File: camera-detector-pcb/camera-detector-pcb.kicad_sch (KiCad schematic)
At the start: 29 parts, among them J1 Conn_01x07, J2 Conn_01x07, J3 Conn_01x04, Q1 PN2222A, SW1 SW_Push, SW2 SW_Push, SW3 SW_Wuerth_450301014042, SW4 SW_Push, U1 74AHCT125

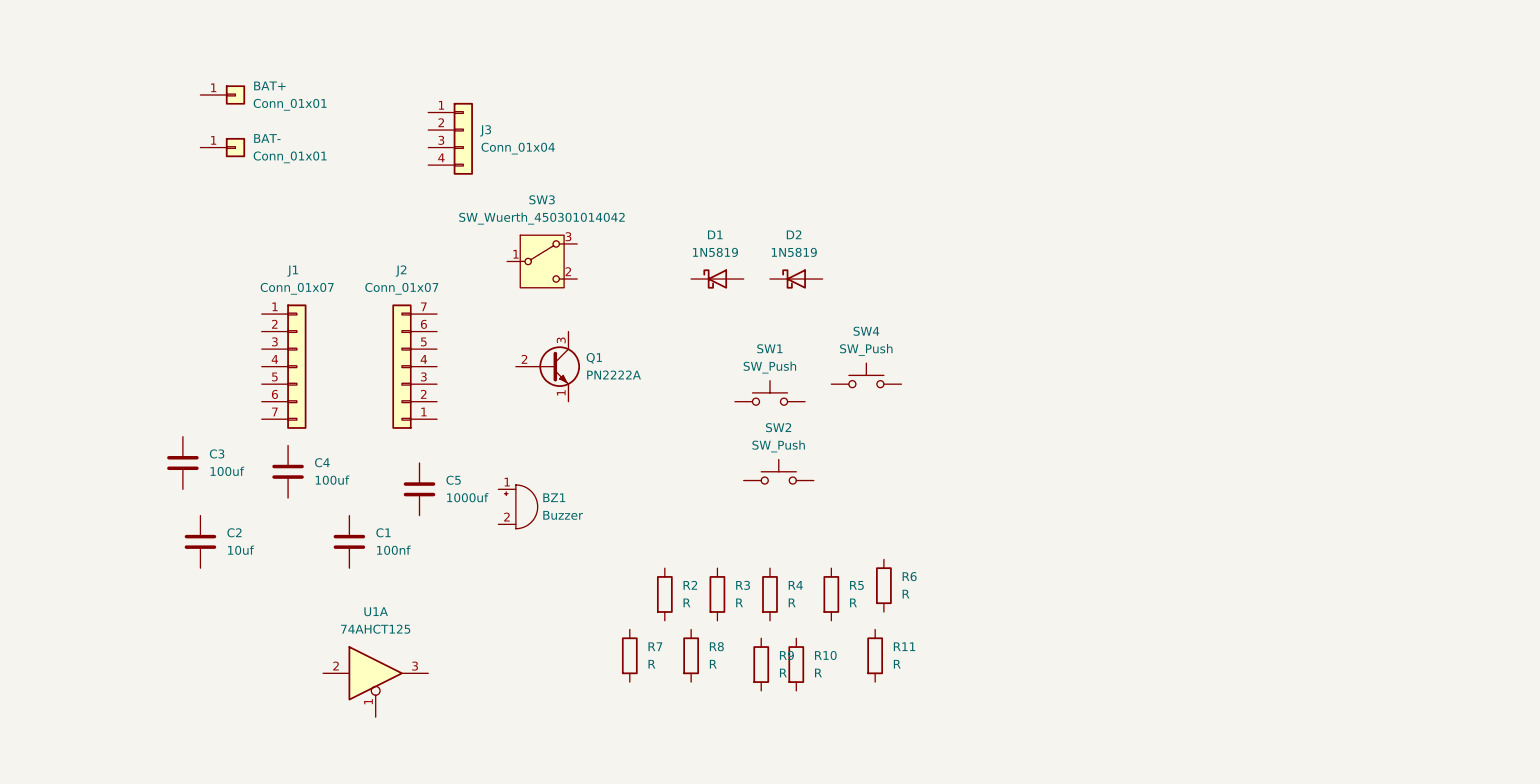
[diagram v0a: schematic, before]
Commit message: completed schematic
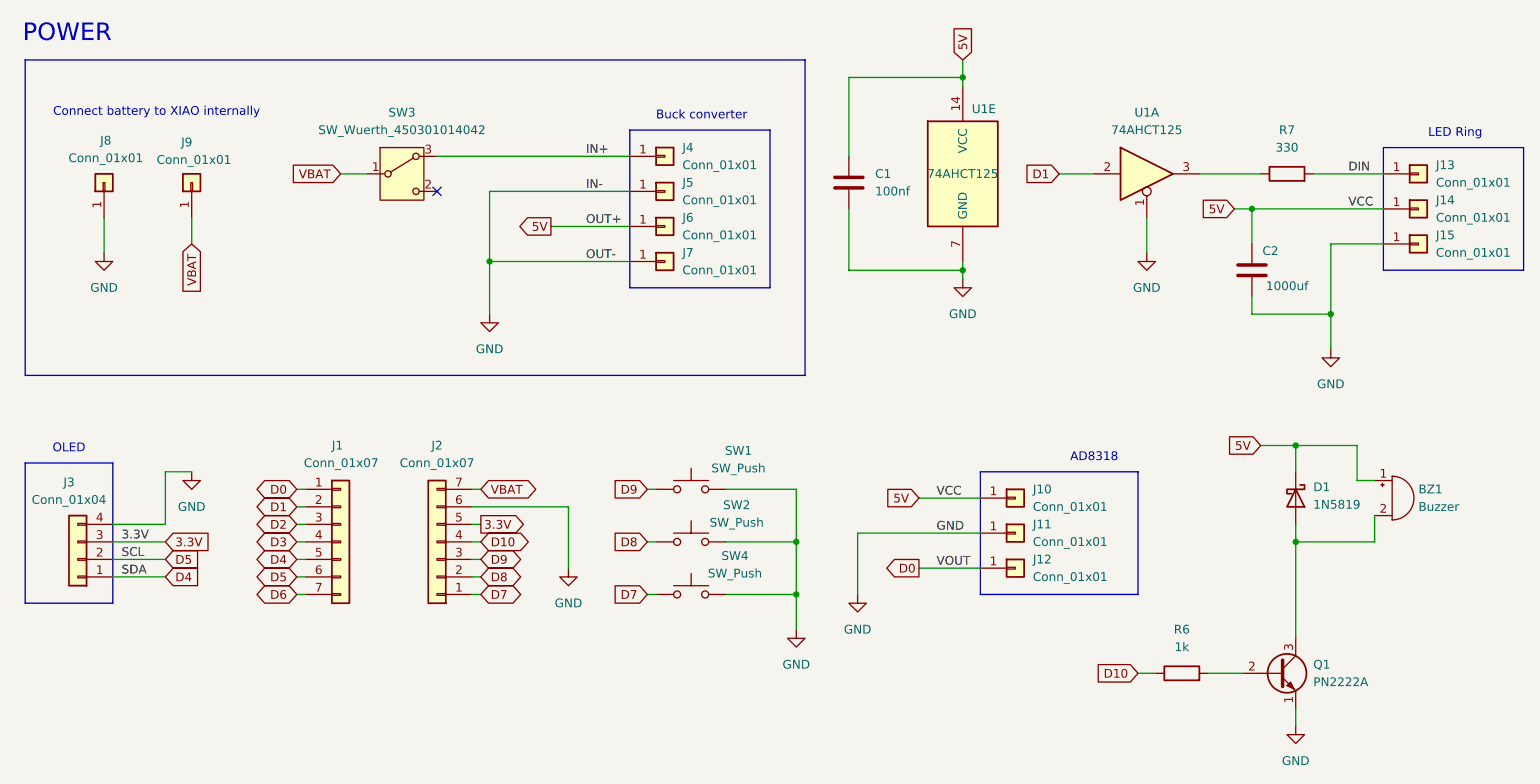
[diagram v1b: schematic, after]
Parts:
- removed C3, C4: 100uf, Capacitor_THT:C_Radial_D5.0mm_H7.0mm_P2.00mm, symbol Device:C
- removed C5: 1000uf, Capacitor_THT:C_Radial_D8.0mm_H11.5mm_P3.50mm, symbol Device:C
- removed D2: 1N5819, Diode_THT:D_DO-41_SOD81_P10.16mm_Horizontal, symbol Diode:1N5819
- removed R10, R11, R2, R3, R4, R5, R8, R9: R, Resistor_THT:R_Axial_DIN0207_L6.3mm_D2.5mm_P15.24mm_Horizontal, symbol Device:R
- added J10, J11, J12, J13, J14, J15, J4, J5, J6, J7: Conn_01x01, symbol Connector_Generic:Conn_01x01
- added unit 5 of U1
- C1: footprint Capacitor_THT:C_Disc_D4.7mm_W2.5mm_P5.00mm -> Capacitor_THT:C_Disc_D3.0mm_W1.6mm_P2.50mm
- C2: value 10uf -> 1000uf; footprint Capacitor_THT:C_Radial_D8.0mm_H7.0mm_P3.50mm -> Capacitor_THT:CP_Radial_D10.0mm_P5.00mm
- R6: value R -> 1k
- R7: value R -> 330
- U1: footprint Package_DIP:DIP-14_W7.62mm -> (none)
- renumbered BAT- to J8, BAT+ to J9
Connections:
- net VBAT: now reaches SW3.1 (B)
- net VBAT: now also J2.7 (Pin_7), J9.1 (Pin_1)
- net IN+: now reaches SW3.3 (A)
- net IN+: now also J4.1 (Pin_1)
- net 5V: now reaches C2.1
- net 5V: now also BZ1.1 (+), C1.1, D1.1 (K), J10.1 (Pin_1), J14.1 (Pin_1), J6.1 (Pin_1), U1.14 (VCC)
- net GND: now reaches C2.2
- net GND: now also C1.2, J2.6 (Pin_6), J3.4 (Pin_4), J8.1 (Pin_1), Q1.1 (E), SW1.2, SW2.2, SW4.2, U1.1, J11.1 (Pin_1), J15.1 (Pin_1), J5.1 (Pin_1), J7.1 (Pin_1), U1.7 (GND)
- net at R7.1: now also U1.3
- net DIN: now reaches R7.2
- net DIN: now also J13.1 (Pin_1)
- net D7: now reaches SW4.1
- net D7: now also J2.1 (Pin_1)
- net D4: now reaches J3.1 (Pin_1)
- net D4: now also J1.5 (Pin_5)
- net D5: now reaches J3.2 (Pin_2)
- net D5: now also J1.6 (Pin_6)
- net 3.3V: now reaches J3.3 (Pin_3)
- net 3.3V: now also J2.5 (Pin_5)
- net D1: now reaches U1.2
- net D1: now also J1.2 (Pin_2)
- net D0: now reaches J1.1 (Pin_1)
- net D0: now also J12.1 (Pin_1)
- net D2: now reaches J1.3 (Pin_3)
- net D3: now reaches J1.4 (Pin_4)
- net D6: now reaches J1.7 (Pin_7)
- net at D1.2 (A): now also BZ1.2 (-), Q1.3 (C)
- net D8: now reaches J2.2 (Pin_2)
- net D8: now also SW2.1
- net D9: now reaches J2.3 (Pin_3)
- net D9: now also SW1.1
- net D10: now reaches J2.4 (Pin_4)
- net D10: now also R6.1
- net at Q1.2 (B): now also R6.2
- no-connect marks 0 -> 1
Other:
- note added: "AD8318"
- note added: "Buck converter"
- note added: "Connect battery to XIAO internally"
- note added: "LED Ring"
- note added: "OLED"
- note added: "POWER"
- moved on the sheet: BZ1, D1, J1, J2, J3, J8, J9, Q1, R6, SW1, SW2, SW3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
